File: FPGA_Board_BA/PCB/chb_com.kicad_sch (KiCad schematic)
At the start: 58 parts, among them J1201 Plug_Terminal_2x12pin, J1202 Plug_Terminal_2x12pin, J1203 Box_Header_6pin, J1204 Box_Header_6pin, J1205 Box_Header_6pin, J1206 Box_Header_6pin, J1401 Plug_Terminal_2x12pin, J1402 Plug_Terminal_2x12pin, J1403 Plug_Terminal_2x12pin, J1404 Plug_Terminal_2x12pin

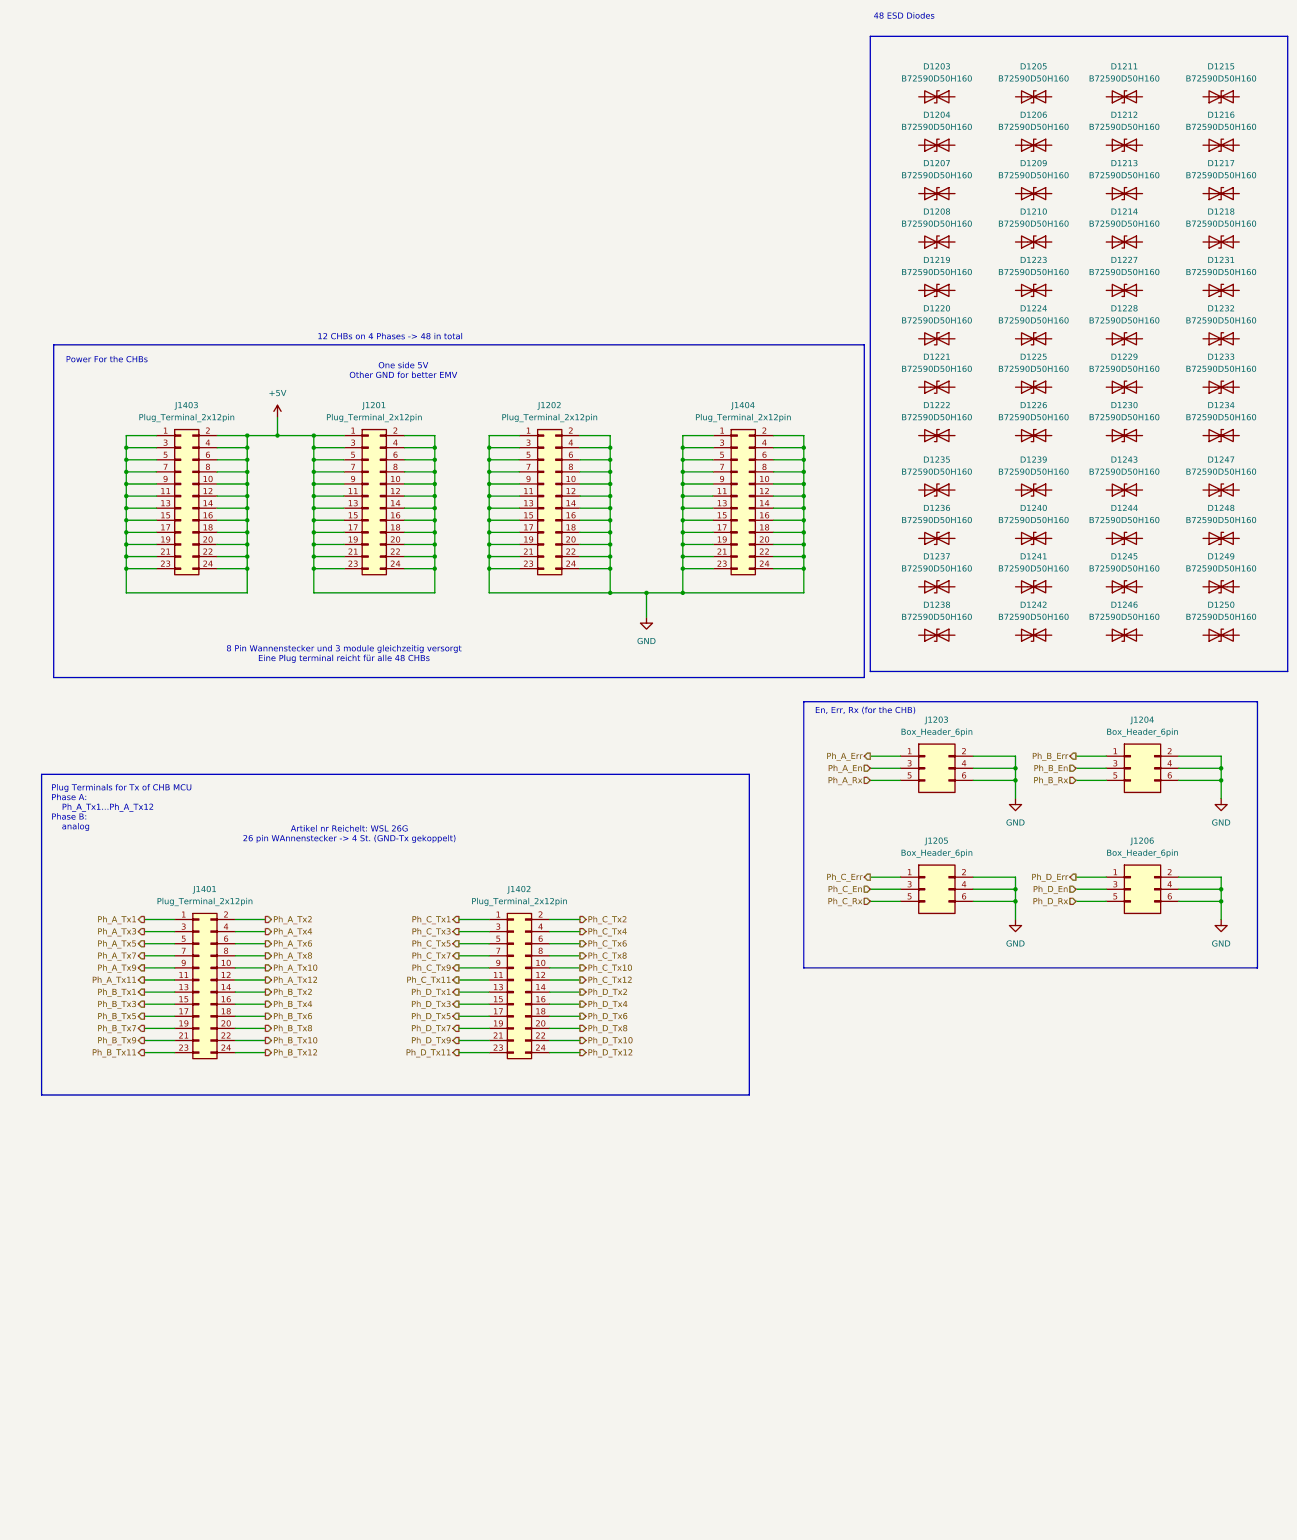
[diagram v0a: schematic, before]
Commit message: lot of work
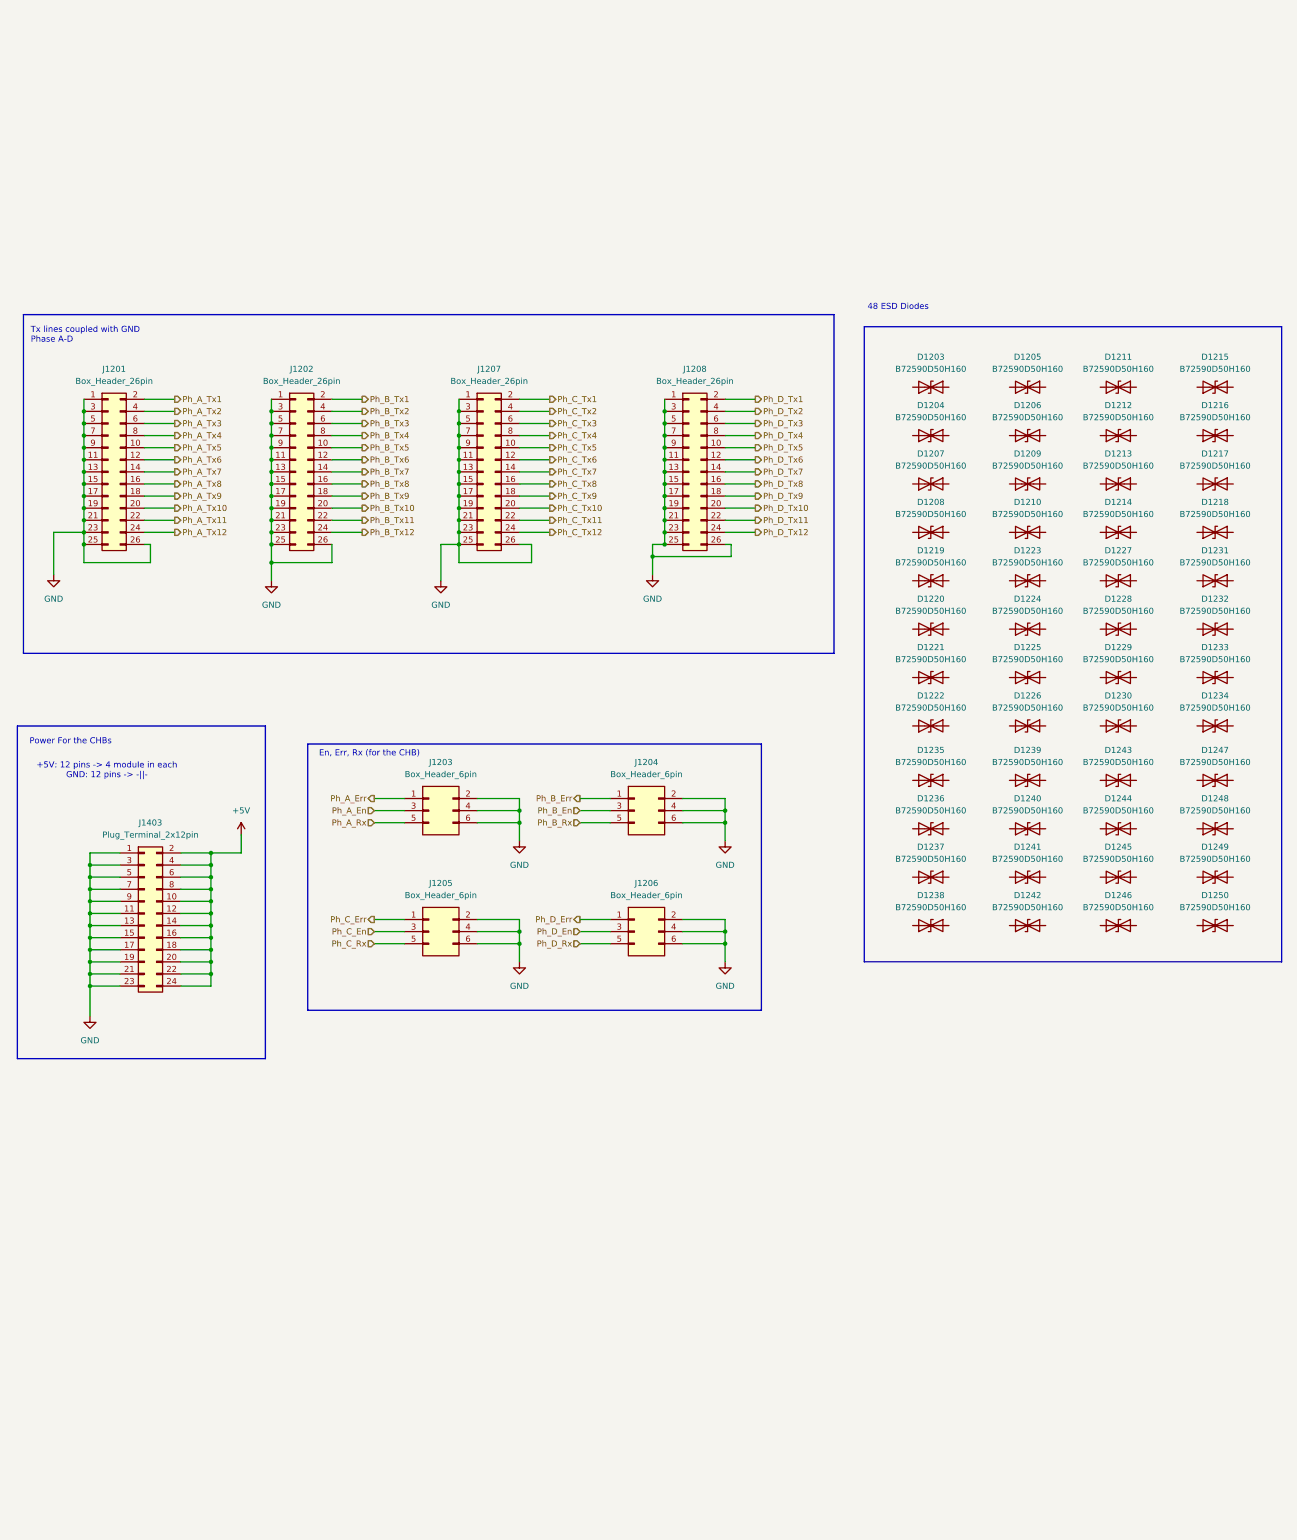
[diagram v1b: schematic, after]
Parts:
- removed J1201, J1202, J1401, J1402, J1404: Plug_Terminal_2x12pin, MYLIB_Misc:DMCV 1,5_12-G1F-3,5-LR P20THR, symbol MYLIB_Misc:Plug_Terminal_2x12pin
- added J1201, J1202, J1207, J1208: Box_Header_26pin, Connector_IDC:IDC-Header_2x13_P2.54mm_Vertical, symbol MYLIB_Misc:Box_Header_26pin
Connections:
- net +5V: no longer J1403.1, J1403.11, J1403.13, J1403.15, J1403.17, J1403.19, J1403.21, J1403.23, J1403.3, J1403.5, J1403.7, J1403.9
- net GND: now also J1403.1, J1403.11, J1403.13, J1403.15, J1403.17, J1403.19, J1403.21, J1403.23, J1403.3, J1403.5, J1403.7, J1403.9, J1201.1 (Pin_1), J1201.11 (Pin_11), J1201.13 (Pin_13), J1201.15 (Pin_15), J1201.17 (Pin_17), J1201.19 (Pin_19), J1201.21 (Pin_21), J1201.23 (Pin_23), J1201.25 (Pin_25), J1201.26 (Pin_26), J1201.3 (Pin_3), J1201.5 (Pin_5), J1201.7 (Pin_7), J1201.9 (Pin_9), J1202.1 (Pin_1), J1202.11 (Pin_11), J1202.13 (Pin_13), J1202.15 (Pin_15), J1202.17 (Pin_17), J1202.19 (Pin_19), J1202.21 (Pin_21), J1202.23 (Pin_23), J1202.25 (Pin_25), J1202.26 (Pin_26), J1202.3 (Pin_3), J1202.5 (Pin_5), J1202.7 (Pin_7), J1202.9 (Pin_9), J1207.1 (Pin_1), J1207.11 (Pin_11), J1207.13 (Pin_13), J1207.15 (Pin_15), J1207.17 (Pin_17), J1207.19 (Pin_19), J1207.21 (Pin_21), J1207.23 (Pin_23), J1207.25 (Pin_25), J1207.26 (Pin_26), J1207.3 (Pin_3), J1207.5 (Pin_5), J1207.7 (Pin_7), J1207.9 (Pin_9), J1208.1 (Pin_1), J1208.11 (Pin_11), J1208.13 (Pin_13), J1208.15 (Pin_15), J1208.17 (Pin_17), J1208.19 (Pin_19), J1208.21 (Pin_21), J1208.23 (Pin_23), J1208.25 (Pin_25), J1208.26 (Pin_26), J1208.3 (Pin_3), J1208.5 (Pin_5), J1208.7 (Pin_7), J1208.9 (Pin_9)
- net Ph_A_Tx1: now also J1201.2 (Pin_2)
- net Ph_A_Tx10: now also J1201.20 (Pin_20)
- net Ph_A_Tx11: now also J1201.22 (Pin_22)
- net Ph_A_Tx12: now also J1201.24 (Pin_24)
- net Ph_A_Tx2: now also J1201.4 (Pin_4)
- net Ph_A_Tx3: now also J1201.6 (Pin_6)
- net Ph_A_Tx4: now also J1201.8 (Pin_8)
- net Ph_A_Tx5: now also J1201.10 (Pin_10)
- net Ph_A_Tx6: now also J1201.12 (Pin_12)
- net Ph_A_Tx7: now also J1201.14 (Pin_14)
- net Ph_A_Tx8: now also J1201.16 (Pin_16)
- net Ph_A_Tx9: now also J1201.18 (Pin_18)
- net Ph_B_Tx1: now also J1202.2 (Pin_2)
- net Ph_B_Tx10: now also J1202.20 (Pin_20)
- net Ph_B_Tx11: now also J1202.22 (Pin_22)
- net Ph_B_Tx12: now also J1202.24 (Pin_24)
- net Ph_B_Tx2: now also J1202.4 (Pin_4)
- net Ph_B_Tx3: now also J1202.6 (Pin_6)
- net Ph_B_Tx4: now also J1202.8 (Pin_8)
- net Ph_B_Tx5: now also J1202.10 (Pin_10)
- net Ph_B_Tx6: now also J1202.12 (Pin_12)
- net Ph_B_Tx7: now also J1202.14 (Pin_14)
- net Ph_B_Tx8: now also J1202.16 (Pin_16)
- net Ph_B_Tx9: now also J1202.18 (Pin_18)
- net Ph_C_Tx1: now also J1207.2 (Pin_2)
- net Ph_C_Tx10: now also J1207.20 (Pin_20)
- net Ph_C_Tx11: now also J1207.22 (Pin_22)
- net Ph_C_Tx12: now also J1207.24 (Pin_24)
- net Ph_C_Tx2: now also J1207.4 (Pin_4)
- net Ph_C_Tx3: now also J1207.6 (Pin_6)
- net Ph_C_Tx4: now also J1207.8 (Pin_8)
- net Ph_C_Tx5: now also J1207.10 (Pin_10)
- net Ph_C_Tx6: now also J1207.12 (Pin_12)
- net Ph_C_Tx7: now also J1207.14 (Pin_14)
- net Ph_C_Tx8: now also J1207.16 (Pin_16)
- net Ph_C_Tx9: now also J1207.18 (Pin_18)
- net Ph_D_Tx1: now also J1208.2 (Pin_2)
- net Ph_D_Tx10: now also J1208.20 (Pin_20)
- net Ph_D_Tx11: now also J1208.22 (Pin_22)
- net Ph_D_Tx12: now also J1208.24 (Pin_24)
- net Ph_D_Tx2: now also J1208.4 (Pin_4)
- net Ph_D_Tx3: now also J1208.6 (Pin_6)
- net Ph_D_Tx4: now also J1208.8 (Pin_8)
- net Ph_D_Tx5: now also J1208.10 (Pin_10)
- net Ph_D_Tx6: now also J1208.12 (Pin_12)
- net Ph_D_Tx7: now also J1208.14 (Pin_14)
- net Ph_D_Tx8: now also J1208.16 (Pin_16)
- net Ph_D_Tx9: now also J1208.18 (Pin_18)
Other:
- note added: "+5V: 12 pins -> 4 module in each GND: 12 pins -> -||-"
- note added: "Tx lines coupled with GND Phase A-D"
- note removed: "12 CHBs on 4 Phases -> 48 in total"
- note removed: "8 Pin Wannenstecker und 3 module gleichzeitig versorgt Eine Plug terminal reicht für alle 48 CHBs"
- note removed: "Artikel nr Reichelt: WSL 26G 26 pin WAnnenstecker -> 4 St. (GND-Tx gekoppelt)"
- note removed: "One side 5V Other GND for better EMV"
- note removed: "Plug Terminals for Tx of CHB MCU Phase A: Ph_A_Tx1...Ph_A_Tx12 Phase B: analog"
- moved on the sheet: D1203, D1204, D1205, D1206, D1207, D1208, D1209, D1210, D1211, D1212, D1213, D1214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

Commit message: lots of work
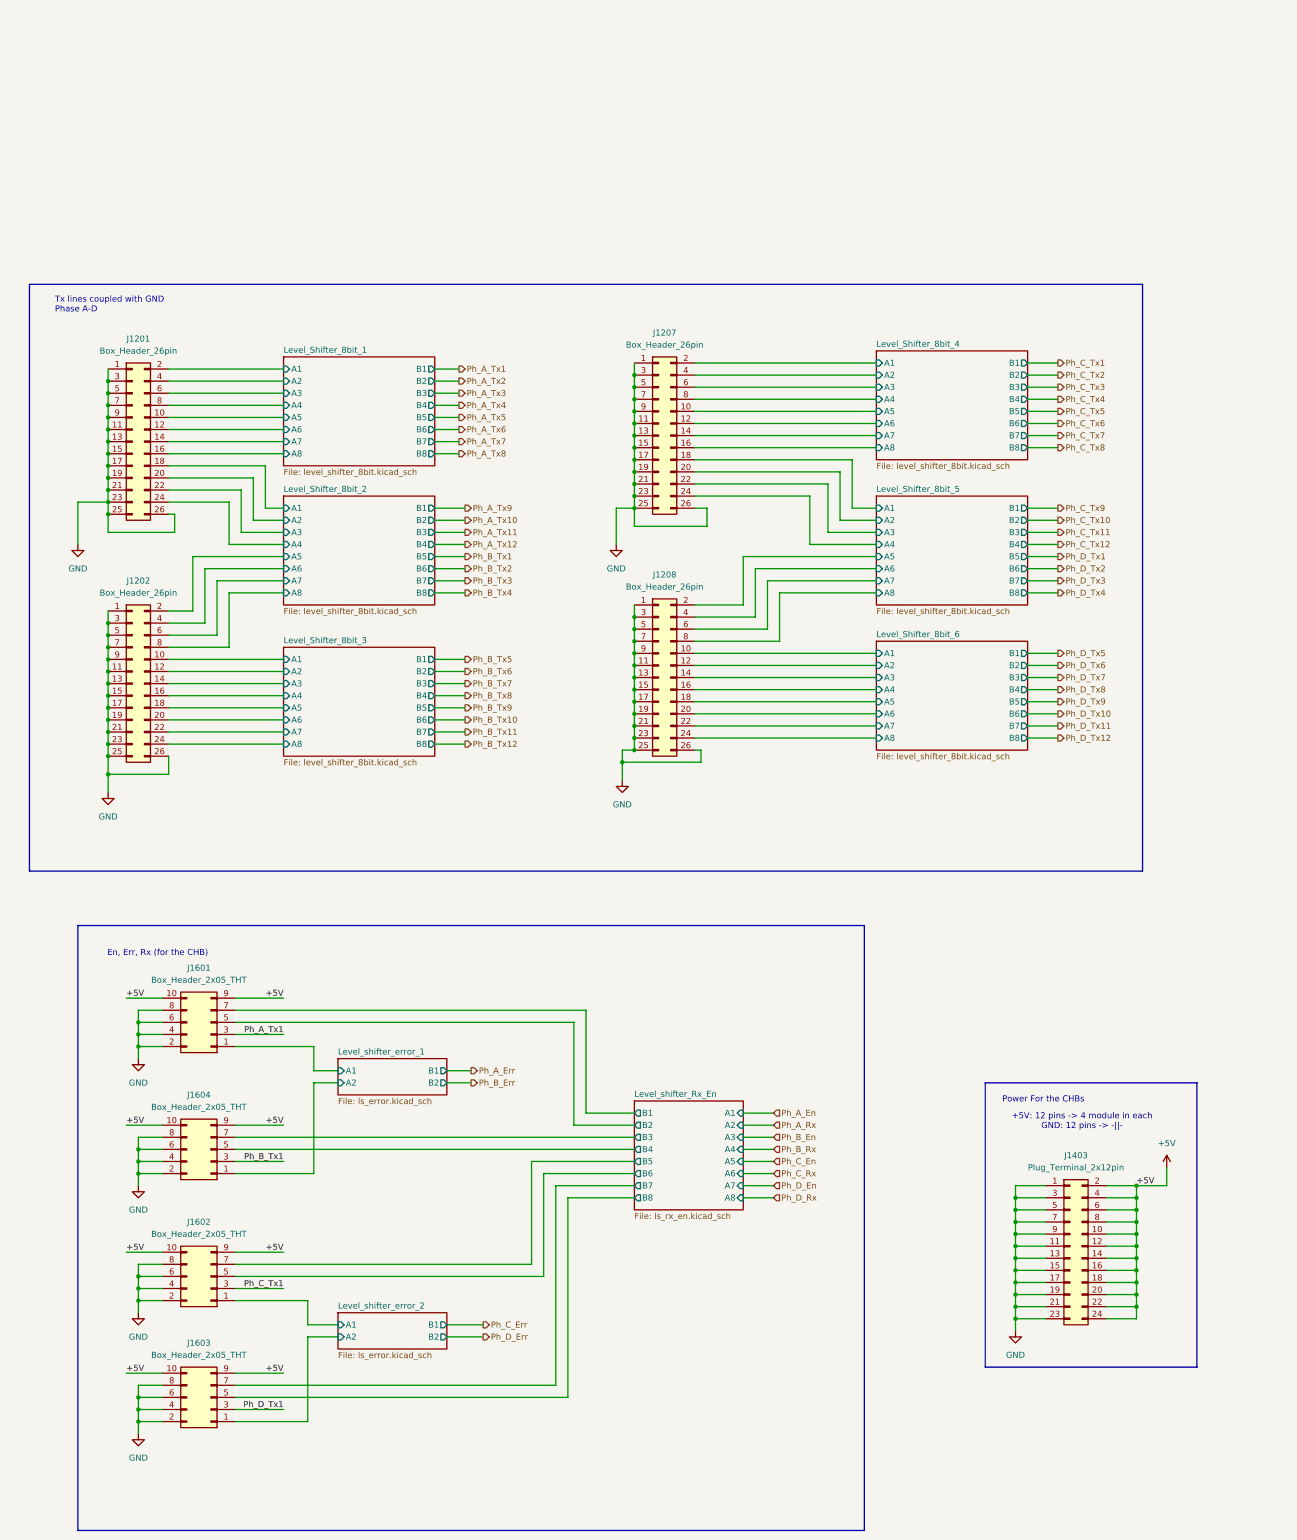
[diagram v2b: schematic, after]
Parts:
- removed D1203, D1204, D1205, D1206, D1207, D1208, D1209, D1210, D1211, D1212, D1213, D1214, D1215, D1216, D1217, D1218, D1219, D1220, D1221, D1222, D1223, D1224, D1225, D1226, D1227, D1228, D1229, D1230, D1231, D1232, D1233, D1234, D1235, D1236, D1237, D1238, D1239, D1240, D1241, D1242, D1243, D1244, D1245, D1246, D1247, D1248, D1249, D1250: B72590D50H160, Capacitor_SMD:C_0402_1005Metric_Pad0.74x0.62mm_HandSolder, symbol MYLIB_Misc:ESD_Diode_5V6
- removed J1203, J1204, J1205, J1206: Box_Header_6pin, Connector_IDC:IDC-Header_2x03_P2.54mm_Vertical, symbol MYLIB_Misc:Box_Header_6pin
- added J1601, J1602, J1603, J1604: Box_Header_2x05_THT, Connector_IDC:IDC-Header_2x05_P2.54mm_Vertical, symbol MYLIB_Misc:Box_Header_10pin
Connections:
- net +5V: now also J1601.10 (Pin_10), J1601.9 (Pin_9), J1602.10 (Pin_10), J1602.9 (Pin_9), J1603.10 (Pin_10), J1603.9 (Pin_9), J1604.10 (Pin_10), J1604.9 (Pin_9)
- net GND: now also J1601.2 (Pin_2), J1601.4 (Pin_4), J1601.6 (Pin_6), J1601.8 (Pin_8), J1602.2 (Pin_2), J1602.4 (Pin_4), J1602.6 (Pin_6), J1602.8 (Pin_8), J1603.2 (Pin_2), J1603.4 (Pin_4), J1603.6 (Pin_6), J1603.8 (Pin_8), J1604.2 (Pin_2), J1604.4 (Pin_4), J1604.6 (Pin_6), J1604.8 (Pin_8)
- net Ph_A_Tx1: now also J1601.3 (Pin_3); no longer J1201.2 (Pin_2)
- net Ph_A_Tx10: no longer J1201.20 (Pin_20)
- net Ph_A_Tx11: no longer J1201.22 (Pin_22)
- net Ph_A_Tx12: no longer J1201.24 (Pin_24)
- net Ph_A_Tx2: no longer J1201.4 (Pin_4)
- net Ph_A_Tx3: no longer J1201.6 (Pin_6)
- net Ph_A_Tx4: no longer J1201.8 (Pin_8)
- net Ph_A_Tx5: no longer J1201.10 (Pin_10)
- net Ph_A_Tx6: no longer J1201.12 (Pin_12)
- net Ph_A_Tx7: no longer J1201.14 (Pin_14)
- net Ph_A_Tx8: no longer J1201.16 (Pin_16)
- net Ph_A_Tx9: no longer J1201.18 (Pin_18)
- net Ph_B_Tx1: now also J1604.3 (Pin_3); no longer J1202.2 (Pin_2)
- net Ph_B_Tx10: no longer J1202.20 (Pin_20)
- net Ph_B_Tx11: no longer J1202.22 (Pin_22)
- net Ph_B_Tx12: no longer J1202.24 (Pin_24)
- net Ph_B_Tx2: no longer J1202.4 (Pin_4)
- net Ph_B_Tx3: no longer J1202.6 (Pin_6)
- net Ph_B_Tx4: no longer J1202.8 (Pin_8)
- net Ph_B_Tx5: no longer J1202.10 (Pin_10)
- net Ph_B_Tx6: no longer J1202.12 (Pin_12)
- net Ph_B_Tx7: no longer J1202.14 (Pin_14)
- net Ph_B_Tx8: no longer J1202.16 (Pin_16)
- net Ph_B_Tx9: no longer J1202.18 (Pin_18)
- net Ph_C_Tx1: now also J1602.3 (Pin_3); no longer J1207.2 (Pin_2)
- net Ph_C_Tx10: no longer J1207.20 (Pin_20)
- net Ph_C_Tx11: no longer J1207.22 (Pin_22)
- net Ph_C_Tx12: no longer J1207.24 (Pin_24)
- net Ph_C_Tx2: no longer J1207.4 (Pin_4)
- net Ph_C_Tx3: no longer J1207.6 (Pin_6)
- net Ph_C_Tx4: no longer J1207.8 (Pin_8)
- net Ph_C_Tx5: no longer J1207.10 (Pin_10)
- net Ph_C_Tx6: no longer J1207.12 (Pin_12)
- net Ph_C_Tx7: no longer J1207.14 (Pin_14)
- net Ph_C_Tx8: no longer J1207.16 (Pin_16)
- net Ph_C_Tx9: no longer J1207.18 (Pin_18)
- net Ph_D_Tx1: now also J1603.3 (Pin_3); no longer J1208.2 (Pin_2)
- net Ph_D_Tx10: no longer J1208.20 (Pin_20)
- net Ph_D_Tx11: no longer J1208.22 (Pin_22)
- net Ph_D_Tx12: no longer J1208.24 (Pin_24)
- net Ph_D_Tx2: no longer J1208.4 (Pin_4)
- net Ph_D_Tx3: no longer J1208.6 (Pin_6)
- net Ph_D_Tx4: no longer J1208.8 (Pin_8)
- net Ph_D_Tx5: no longer J1208.10 (Pin_10)
- net Ph_D_Tx6: no longer J1208.12 (Pin_12)
- net Ph_D_Tx7: no longer J1208.14 (Pin_14)
- net Ph_D_Tx8: no longer J1208.16 (Pin_16)
- net Ph_D_Tx9: no longer J1208.18 (Pin_18)
- new net Level_Shifter_8bit_1/A1: J1201.2 (Pin_2)
- new net Level_Shifter_8bit_1/A2: J1201.4 (Pin_4)
- new net Level_Shifter_8bit_1/A3: J1201.6 (Pin_6)
- new net Level_Shifter_8bit_1/A4: J1201.8 (Pin_8)
- new net Level_Shifter_8bit_1/A5: J1201.10 (Pin_10)
- new net Level_Shifter_8bit_1/A6: J1201.12 (Pin_12)
- new net Level_Shifter_8bit_1/A7: J1201.14 (Pin_14)
- new net Level_Shifter_8bit_1/A8: J1201.16 (Pin_16)
- new net Level_Shifter_8bit_2/A1: J1201.18 (Pin_18)
- new net Level_Shifter_8bit_2/A2: J1201.20 (Pin_20)
- new net Level_Shifter_8bit_2/A3: J1201.22 (Pin_22)
- new net Level_Shifter_8bit_2/A4: J1201.24 (Pin_24)
- new net Level_Shifter_8bit_2/A5: J1202.2 (Pin_2)
- new net Level_Shifter_8bit_2/A6: J1202.4 (Pin_4)
- new net Level_Shifter_8bit_2/A7: J1202.6 (Pin_6)
- new net Level_Shifter_8bit_2/A8: J1202.8 (Pin_8)
- new net Level_Shifter_8bit_3/A1: J1202.10 (Pin_10)
- new net Level_Shifter_8bit_3/A2: J1202.12 (Pin_12)
- new net Level_Shifter_8bit_3/A3: J1202.14 (Pin_14)
- new net Level_Shifter_8bit_3/A4: J1202.16 (Pin_16)
- new net Level_Shifter_8bit_3/A5: J1202.18 (Pin_18)
- new net Level_Shifter_8bit_3/A6: J1202.20 (Pin_20)
- new net Level_Shifter_8bit_3/A7: J1202.22 (Pin_22)
- new net Level_Shifter_8bit_3/A8: J1202.24 (Pin_24)
- new net Level_Shifter_8bit_4/A1: J1207.2 (Pin_2)
- new net Level_Shifter_8bit_4/A2: J1207.4 (Pin_4)
- new net Level_Shifter_8bit_4/A3: J1207.6 (Pin_6)
- new net Level_Shifter_8bit_4/A4: J1207.8 (Pin_8)
- new net Level_Shifter_8bit_4/A5: J1207.10 (Pin_10)
- new net Level_Shifter_8bit_4/A6: J1207.12 (Pin_12)
- new net Level_Shifter_8bit_4/A7: J1207.14 (Pin_14)
- new net Level_Shifter_8bit_4/A8: J1207.16 (Pin_16)
- new net Level_Shifter_8bit_5/A1: J1207.18 (Pin_18)
- new net Level_Shifter_8bit_5/A2: J1207.20 (Pin_20)
- new net Level_Shifter_8bit_5/A3: J1207.22 (Pin_22)
- new net Level_Shifter_8bit_5/A4: J1207.24 (Pin_24)
- new net Level_Shifter_8bit_5/A5: J1208.2 (Pin_2)
- new net Level_Shifter_8bit_5/A6: J1208.4 (Pin_4)
- new net Level_Shifter_8bit_5/A7: J1208.6 (Pin_6)
- new net Level_Shifter_8bit_5/A8: J1208.8 (Pin_8)
- new net Level_Shifter_8bit_6/A1: J1208.10 (Pin_10)
- new net Level_Shifter_8bit_6/A2: J1208.12 (Pin_12)
- new net Level_Shifter_8bit_6/A3: J1208.14 (Pin_14)
- new net Level_Shifter_8bit_6/A4: J1208.16 (Pin_16)
- new net Level_Shifter_8bit_6/A5: J1208.18 (Pin_18)
- new net Level_Shifter_8bit_6/A6: J1208.20 (Pin_20)
- new net Level_Shifter_8bit_6/A7: J1208.22 (Pin_22)
- new net Level_Shifter_8bit_6/A8: J1208.24 (Pin_24)
- new net Level_shifter_Rx_En/B1: J1601.7 (Pin_7)
- new net Level_shifter_Rx_En/B2: J1601.5 (Pin_5)
- new net Level_shifter_Rx_En/B3: J1604.7 (Pin_7)
- new net Level_shifter_Rx_En/B4: J1604.5 (Pin_5)
- new net Level_shifter_Rx_En/B5: J1602.7 (Pin_7)
- new net Level_shifter_Rx_En/B6: J1602.5 (Pin_5)
- new net Level_shifter_Rx_En/B7: J1603.7 (Pin_7)
- new net Level_shifter_Rx_En/B8: J1603.5 (Pin_5)
- new net Level_shifter_error_1/A1: J1601.1 (Pin_1)
- new net Level_shifter_error_1/A2: J1604.1 (Pin_1)
- new net Level_shifter_error_2/A1: J1602.1 (Pin_1)
- new net Level_shifter_error_2/A2: J1603.1 (Pin_1)
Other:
- added sheet Level_Shifter_8bit_1 (level_shifter_8bit.kicad_sch)
- added sheet Level_Shifter_8bit_2 (level_shifter_8bit.kicad_sch)
- added sheet Level_Shifter_8bit_3 (level_shifter_8bit.kicad_sch)
- added sheet Level_Shifter_8bit_4 (level_shifter_8bit.kicad_sch)
- added sheet Level_Shifter_8bit_5 (level_shifter_8bit.kicad_sch)
- added sheet Level_Shifter_8bit_6 (level_shifter_8bit.kicad_sch)
- added sheet Level_shifter_Rx_En (ls_rx_en.kicad_sch)
- added sheet Level_shifter_error_1 (ls_error.kicad_sch)
- added sheet Level_shifter_error_2 (ls_error.kicad_sch)
- note removed: "48 ESD Diodes"
- moved on the sheet: J1201, J1202, J1207, J1208, J1403
